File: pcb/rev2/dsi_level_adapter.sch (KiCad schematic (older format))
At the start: 6 parts

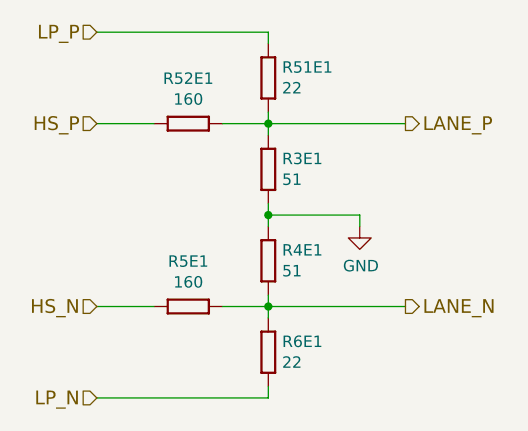
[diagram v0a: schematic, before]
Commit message: pcb wip
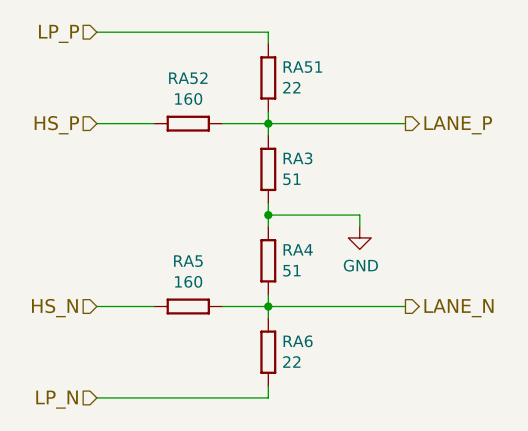
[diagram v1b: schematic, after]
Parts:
- RA3: renamed from R3A1; footprint RESC1608X55N -> Resistors SMD:RESC1608X55N
- RA4: renamed from R4A1; footprint RESC1608X55N -> Resistors SMD:RESC1608X55N
- RA5: renamed from R5A1; footprint RESC1608X55N -> Resistors SMD:RESC1608X55N
- RA51: renamed from R51A1; footprint RESC1608X55N -> Resistors SMD:RESC1608X55N; Fieldname (none) -> Value
- RA52: renamed from R52A1; footprint RESC1608X55N -> Resistors SMD:RESC1608X55N
- RA6: renamed from R6A; footprint RESC1608X55N -> Resistors SMD:RESC1608X55N
